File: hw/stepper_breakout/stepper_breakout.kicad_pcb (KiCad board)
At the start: 2 copper layers, 72.4 x 132.1 mm, 56 parts, among them P1 X_HOME, P10 A, P11 Y, P12 POWER_IN, P13 B, P14 X, P15 CONN_02X25, P2 Y_HOME, P3 Z_HOME, P4 A_HOME, P5 B_HOME, P6 TOOL_PROBE, P7 PIECE_PROBE, P8 E_STOP, P9 Z, U1 NSI45030, U2 NSI45030, U3 NSI45030, U4 NSI45030, U5 NSI45030, U6 NSI45030, U7 NSI45030, U8 NSI45030

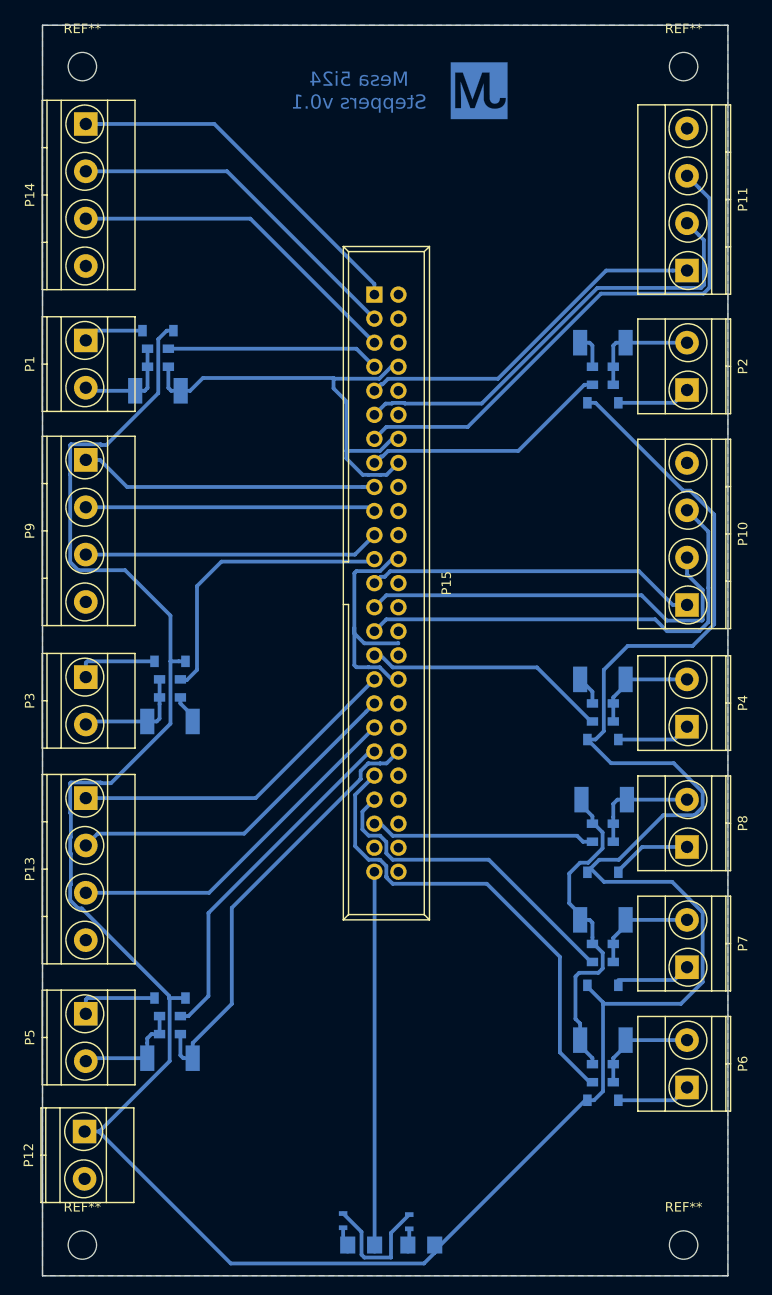
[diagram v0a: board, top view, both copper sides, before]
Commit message: Tweak power and breakout boards a little
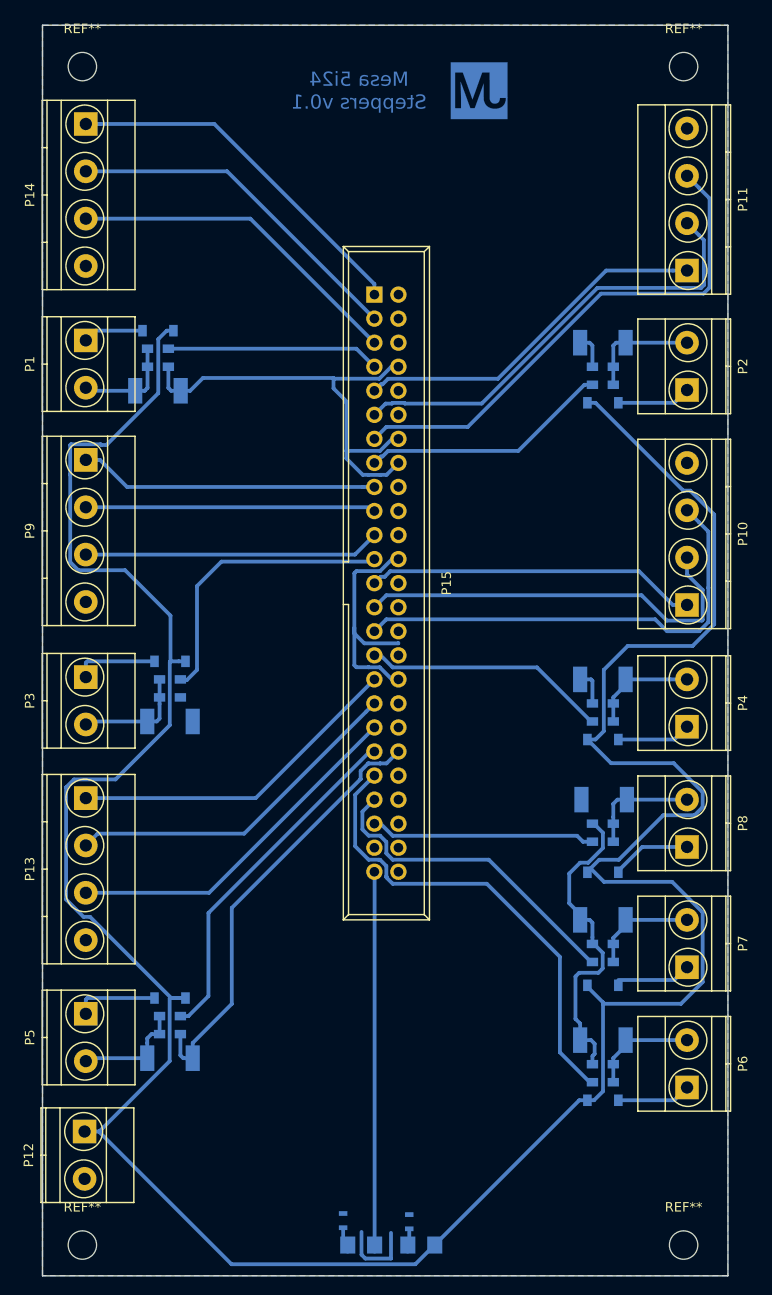
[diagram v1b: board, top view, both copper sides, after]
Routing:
- net GND: track 181.6 -> 173.5 mm
- net +12V: track 312.6 -> 314.4 mm
